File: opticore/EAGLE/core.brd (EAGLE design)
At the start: 100.3 x 80 mm, 67 parts, among them IC2 MC33269T-5.0, J1 POWER_JACKSLT, Q1 2N3904, Q2 2N3904, Q3 2N3904, Q4 2N3904, Q5 2N3904, Q6 2N3904, Q7 2N3904, X1 FFKV8

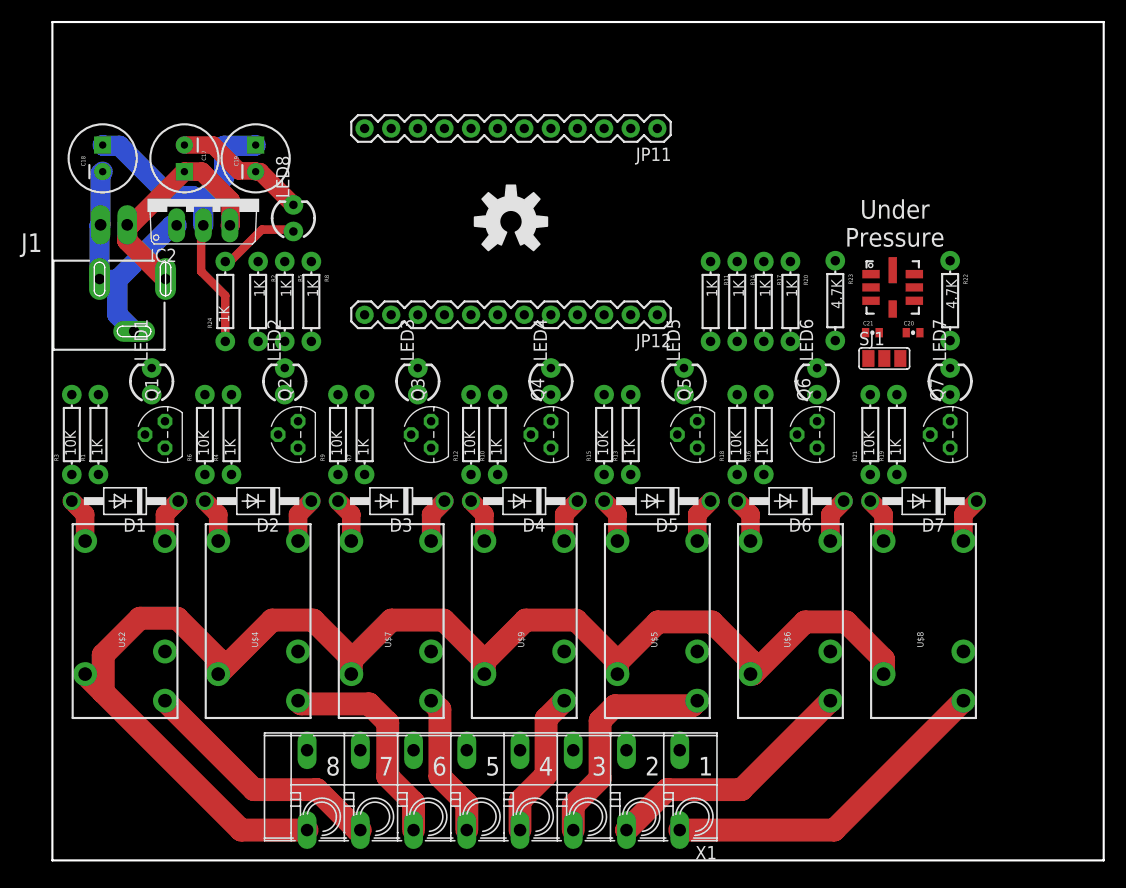
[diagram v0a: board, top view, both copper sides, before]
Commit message: Under Pressure
Adding a bit of personality to the board. Essentially have a good
layout. Still need to do the changes from 2 commits ago.
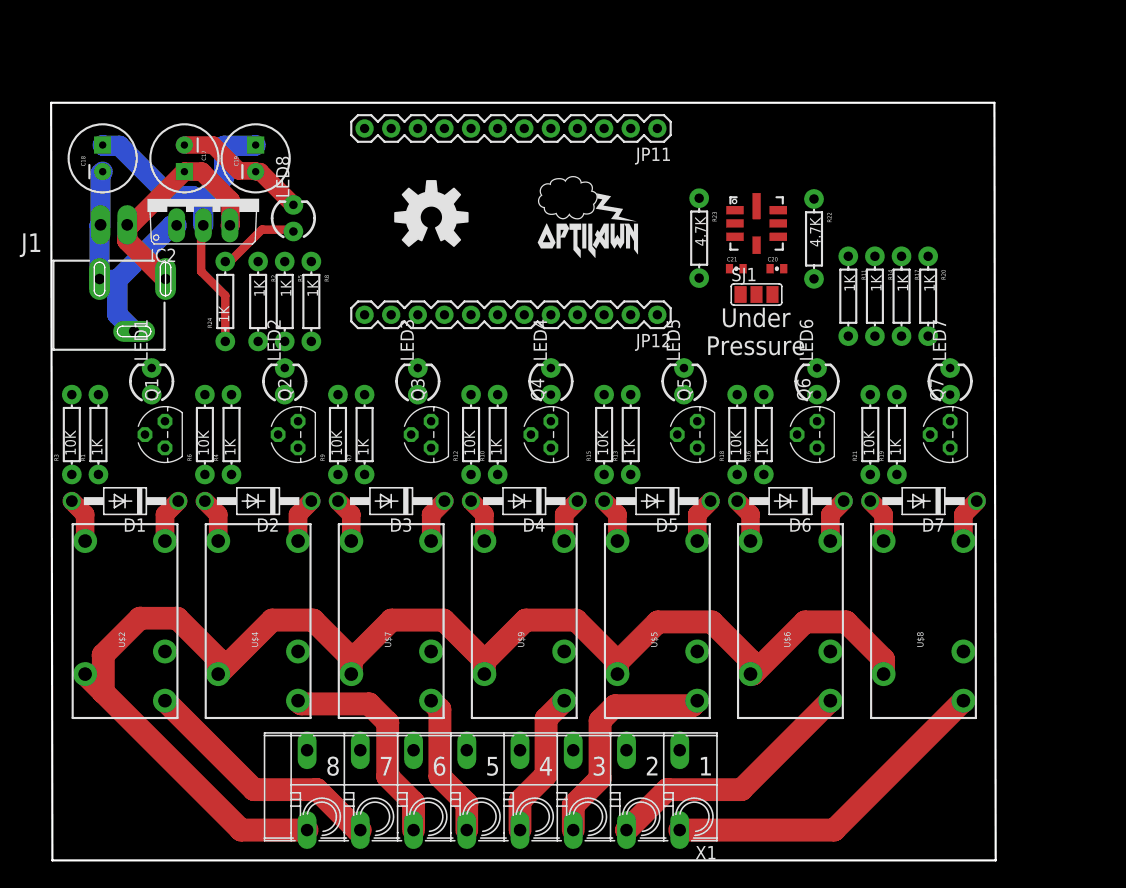
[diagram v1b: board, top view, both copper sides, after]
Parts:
- moved C20 14.4 mm to (69.1, 56.5)
- moved C21 14.4 mm to (65.3, 56.5)
- moved U$3 14.4 mm to (67.2, 60.8)
- moved R23 14.3 mm to (61.7, 59.4)
- moved R22 14.3 mm to (72.7, 59.3)
- moved SJ1 13.6 mm to (67.2, 54.0)
- moved R11 13.2 mm to (76.0, 53.8)
- moved R14 13.2 mm to (78.5, 53.8)
- moved R17 13.2 mm to (81.0, 53.8)
- moved R20 13.2 mm to (83.6, 53.8)
- moved LOGO2 7.61 mm to (36.2, 61.4)
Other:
- board size 100.3 x 80 mm -> 90.1 x 72.3 mm
- board text added: "D:/Users/Scott/Documents/GitHub/optisprk/eagle_custom_icon.bmp"
